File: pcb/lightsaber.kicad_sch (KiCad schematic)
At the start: 66 parts, among them IC1 BMI055, J1 2012670005, J2 Screw_Terminal_01x05, J3 ESP32 Prog, J4 ESP32 JTAG, J5 Conn_01x02, J6 Conn_01x06, Q1 PMOS, Q2 NPN, SW1 SW_Push, SW2 SW_Push, U1 ME6211A33PG-N, U2 ESP32-S3-WROOM-1, U3 ACS725xLCTR-10AU, U4 BQ21040DBVR, U5 5994, U6 MAX17048G+T10, U7 AHT20

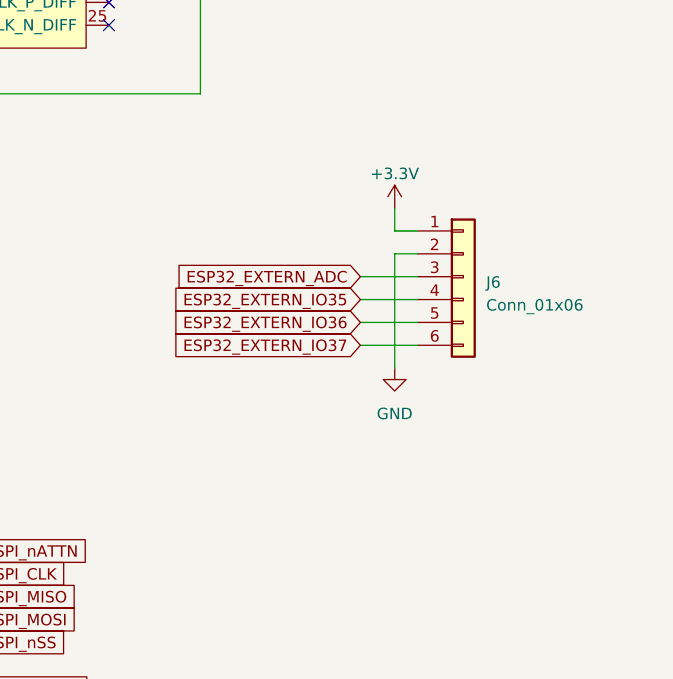
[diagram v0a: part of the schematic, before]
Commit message: Tidying up traces
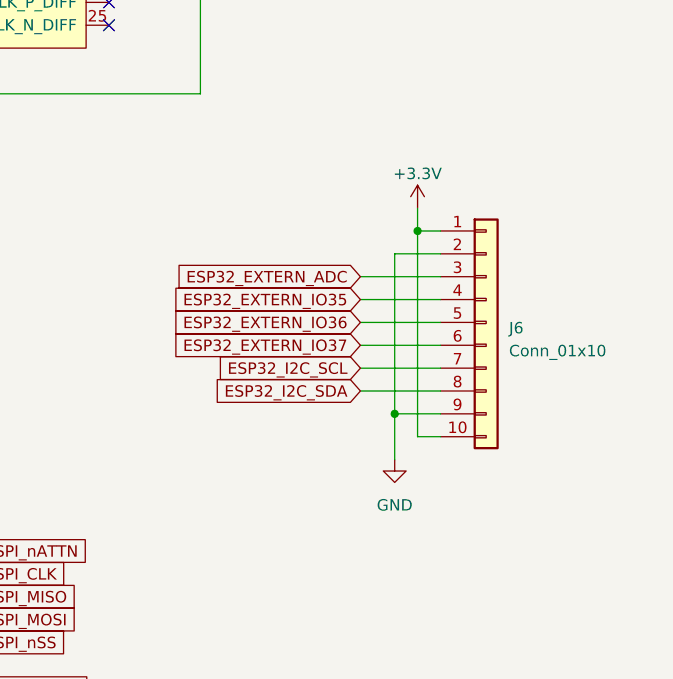
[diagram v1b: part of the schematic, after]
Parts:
- removed J6: Conn_01x06, Connector_PinHeader_2.54mm:PinHeader_1x06_P2.54mm_Vertical, symbol Connector_Generic:Conn_01x06
- added J6: Conn_01x10, Connector_PinHeader_2.54mm:PinHeader_1x10_P2.54mm_Vertical, symbol Connector_Generic:Conn_01x10
- SW1, SW2: LCSC C318884 -> C492878
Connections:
- net +3.3V: now also J6.1 (Pin_1), J6.10 (Pin_10)
- net ESP32_EXTERN_ADC: now also J6.3 (Pin_3)
- net ESP32_EXTERN_IO35: now also J6.4 (Pin_4)
- net ESP32_EXTERN_IO36: now also J6.5 (Pin_5)
- net ESP32_EXTERN_IO37: now also J6.6 (Pin_6)
- net ESP32_I2C_SCL: now also J6.7 (Pin_7)
- net ESP32_I2C_SDA: now also J6.8 (Pin_8)
- net GND: now also J6.2 (Pin_2), J6.9 (Pin_9)
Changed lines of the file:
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@@
   (junction (at 118.11 201.93) (diameter 0) (color 0 0 0 0)
   )
+  (junction (at 544.83 158.75) (diameter 0) (color 0 0 0 0)
+  )
   (junction (at 21.59 44.45) (diameter 0) (color 0 0 0 0)
   )
@@
   (junction (at 387.35 44.45) (diameter 0) (color 0 0 0 0)
   )
+  (junction (at 547.37 138.43) (diameter 0) (color 0 0 0 0)
+  )
   (junction (at 466.09 212.09) (diameter 0) (color 0 0 0 0)
   )
@@
     (stroke (width 0) (type default))
   )
-  (wire (pts (xy 544.83 138.43) (xy 547.37 138.43))
+  (wire (pts (xy 547.37 138.43) (xy 549.91 138.43))
     (stroke (width 0) (type default))
   )
@@
     (stroke (width 0) (type default))
   )
-  (wire (pts (xy 544.83 140.97) (xy 544.83 153.67))
+  (wire (pts (xy 544.83 140.97) (xy 544.83 158.75))
     (stroke (width 0) (type default))
   )
@@
     (stroke (width 0) (type default))
   )
-  (wire (pts (xy 544.83 140.97) (xy 547.37 140.97))
+  (wire (pts (xy 544.83 140.97) (xy 549.91 140.97))
     (stroke (width 0) (type default))
   )
@@
     (stroke (width 0) (type default))
   )
+  (wire (pts (xy 541.02 153.67) (xy 549.91 153.67))
+    (stroke (width 0) (type default))
+  )
   (wire (pts (xy 476.25 209.55) (xy 476.25 212.09))
     (stroke (width 0) (type default))
@@
     (stroke (width 0) (type default))
   )
+  (wire (pts (xy 549.91 161.29) (xy 547.37 161.29))
+    (stroke (width 0) (type default))
+  )
   (wire (pts (xy 114.3 261.62) (xy 111.76 261.62))
     (stroke (width 0) (type default))
@@
     (stroke (width 0) (type default))
   )
+  (wire (pts (xy 544.83 158.75) (xy 544.83 163.83))
+    (stroke (width 0) (type default))
+  )
   (wire (pts (xy 104.14 130.81) (xy 107.95 130.81))
     (stroke (width 0) (type default))
@@
     (stroke (width 0) (type default))
   )
-  (wire (pts (xy 541.02 146.05) (xy 547.37 146.05))
+  (wire (pts (xy 541.02 146.05) (xy 549.91 146.05))
     (stroke (width 0) (type default))
   )
@@
     (stroke (width 0) (type default))
   )
-  (wire (pts (xy 541.02 143.51) (xy 547.37 143.51))
+  (wire (pts (xy 541.02 143.51) (xy 549.91 143.51))
     (stroke (width 0) (type default))
   )
@@
     (stroke (width 0) (type default))
   )
+  (wire (pts (xy 547.37 161.29) (xy 547.37 138.43))
+    (stroke (width 0) (type default))
+  )
   (wire (pts (xy 140.97 125.73) (xy 140.97 115.57))
     (stroke (width 0) (type default))
@@
     (stroke (width 0) (type default))
   )
+  (wire (pts (xy 541.02 156.21) (xy 549.91 156.21))
+    (stroke (width 0) (type default))
+  )
   (wire (pts (xy 58.42 123.19) (xy 60.96 123.19))
     (stroke (width 0) (type default))
@@
     (stroke (width 0) (type default))
   )
+  (wire (pts (xy 544.83 158.75) (xy 549.91 158.75))
+    (stroke (width 0) (type default))
+  )
   (wire (pts (xy 513.08 90.17) (xy 528.32 90.17))
     (stroke (width 0) (type default))
@@
     (stroke (width 0) (type default))
   )
-  (wire (pts (xy 541.02 151.13) (xy 547.37 151.13))
+  (wire (pts (xy 541.02 151.13) (xy 549.91 151.13))
     (stroke (width 0) (type default))
   )
@@
     (stroke (width 0) (type default))
   )
-  (wire (pts (xy 541.02 148.59) (xy 547.37 148.59))
+  (wire (pts (xy 541.02 148.59) (xy 549.91 148.59))
     (stroke (width 0) (type default))
   )
@@
     (stroke (width 0) (type default))
   )
-  (wire (pts (xy 544.83 135.89) (xy 544.83 138.43))
+  (wire (pts (xy 547.37 135.89) (xy 547.37 138.43))
     (stroke (width 0) (type default))
   )
@@
     )
   )
+  (global_label "ESP32_I2C_SDA" (shape input) (at 541.02 156.21 180) (fields_autoplaced)
+    (effects (font (size 1.27 1.27)) (justify right))
+    (property "Intersheetrefs" "${INTERSHEET_REFS}" (at 523.4791 156.21 0)
+      (effects (font (size 1.27 1.27)) (justify right) hide)
+    )
+  )
   (global_label "ESP32_BMI_GYRO_2" (shape input) (at 528.32 77.47 0) (fields_autoplaced)
     (effects (font (size 1.27 1.27)) (justify left))
@@
     )
   )
+  (global_label "ESP32_I2C_SCL" (shape input) (at 541.02 153.67 180) (fields_autoplaced)
+    (effects (font (size 1.27 1.27)) (justify right))
+    (property "Intersheetrefs" "${INTERSHEET_REFS}" (at 523.5396 153.67 0)
+      (effects (font (size 1.27 1.27)) (justify right) hide)
+    )
+  )
   (global_label "ESP32_EXTERN_IO37" (shape input) (at 416.56 115.57 180) (fields_autoplaced)
     (effects (font (size 1.27 1.27)) (justify right))
@@
     )
   )
-  (symbol (lib_id "power:+3.3V") (at 544.83 135.89 0) (unit 1)
+  (symbol (lib_id "power:+3.3V") (at 547.37 135.89 0) (unit 1)
     (in_bom yes) (on_board yes) (dnp no) (fields_autoplaced)
-    (property "Reference" "#PWR039" (at 544.83 139.7 0)
+    (property "Reference" "#PWR039" (at 547.37 139.7 0)
       (effects (font (size 1.27 1.27)) hide)
     )
-    (property "Value" "+3.3V" (at 544.83 132.08 0)
+    (property "Value" "+3.3V" (at 547.37 132.08 0)
       (effects (font (size 1.27 1.27)))
     )
-    (property "Footprint" "" (at 544.83 135.89 0)
+    (property "Footprint" "" (at 547.37 135.89 0)
       (effects (font (size 1.27 1.27)) hide)
     )
-    (property "Datasheet" "" (at 544.83 135.89 0)
+    (property "Datasheet" "" (at 547.37 135.89 0)
       (effects (font (size 1.27 1.27)) hide)
     )
@@
     )
   )
-  (symbol (lib_id "power:GND") (at 544.83 153.67 0) (unit 1)
+  (symbol (lib_id "power:GND") (at 544.83 163.83 0) (unit 1)
     (in_bom yes) (on_board yes) (dnp no) (fields_autoplaced)
-    (property "Reference" "#PWR050" (at 544.83 160.02 0)
+    (property "Reference" "#PWR050" (at 544.83 170.18 0)
       (effects (font (size 1.27 1.27)) hide)
     )
-    (property "Value" "GND" (at 544.83 158.75 0)
+    (property "Value" "GND" (at 544.83 168.91 0)
       (effects (font (size 1.27 1.27)))
     )
-    (property "Footprint" "" (at 544.83 153.67 0)
+    (property "Footprint" "" (at 544.83 163.83 0)
       (effects (font (size 1.27 1.27)) hide)
     )
-    (property "Datasheet" "" (at 544.83 153.67 0)
+    (property "Datasheet" "" (at 544.83 163.83 0)
       (effects (font (size 1.27 1.27)) hide)
     )
@@
       (effects (font (size 1.27 1.27)) hide)
     )
-    (property "LCSC" "C318884" (at 189.23 280.67 0)
+    (property "LCSC" "C492878" (at 189.23 280.67 0)
+      (effects (font (size 1.27 1.27)) hide)
+    )
+    (property "Field" "" (at 189.23 280.67 90)
       (effects (font (size 1.27 1.27)) hide)
     )
@@
     )
   )
+  (symbol (lib_id "Connector_Generic:Conn_01x10") (at 554.99 148.59 0) (unit 1)
+    (in_bom yes) (on_board yes) (dnp no) (fields_autoplaced)
+    (property "Reference" "J6" (at 557.53 149.225 0)
+      (effects (font (size 1.27 1.27)) (justify left))
+    )
+    (property "Value" "Conn_01x10" (at 557.53 151.765 0)
+      (effects (font (size 1.27 1.27)) (justify left))
+    )
+    (property "Footprint" "Connector_PinHeader_2.54mm:PinHeader_1x10_P2.54mm_Vertical" (at 554.99 148.59 0)
+      (effects (font (size 1.27 1.27)) hide)
+    )
+    (property "Datasheet" "~" (at 554.99 148.59 0)
+      (effects (font (size 1.27 1.27)) hide)
+    )
+    (pin "1")
+    (pin "10")
+    (pin "2")
+    (pin "3")
+    (pin "4")
+    (pin "5")
+    (pin "6")
+    (pin "7")
+    (pin "8")
+    (pin "9")
+    (instances
+      (project "lightsaber"
+        (path "/480b6f8b-587f-4642-8a87-aec0c171ba44"
+          (reference "J6") (unit 1)
+        )
+      )
+    )
+  )
   (symbol (lib_id "power:+3.3V") (at 316.23 252.73 0) (unit 1)
     (in_bom yes) (on_board yes) (dnp no) (fields_autoplaced)
@@
     )
   )
-  (symbol (lib_id "Connector_Generic:Conn_01x06") (at 552.45 143.51 0) (unit 1)
-    (in_bom yes) (on_board yes) (dnp no) (fields_autoplaced)
-    (property "Reference" "J6" (at 554.99 144.145 0)
-      (effects (font (size 1.27 1.27)) (justify left))
-    )
-    (property "Value" "Conn_01x06" (at 554.99 146.685 0)
-      (effects (font (size 1.27 1.27)) (justify left))
-    )
-    (property "Footprint" "Connector_PinHeader_2.54mm:PinHeader_1x06_P2.54mm_Vertical" (at 552.45 143.51 0)
-      (effects (font (size 1.27 1.27)) hide)
-    )
-    (property "Datasheet" "~" (at 552.45 143.51 0)
-      (effects (font (size 1.27 1.27)) hide)
-    )
-    (pin "1")
-    (pin "2")
-    (pin "3")
-    (pin "4")
-    (pin "5")
-    (pin "6")
-    (instances
-      (project "lightsaber"
-        (path "/480b6f8b-587f-4642-8a87-aec0c171ba44"
-          (reference "J6") (unit 1)
-        )
-      )
-    )
-  )
   (symbol (lib_id "Device:C_Small") (at 140.97 128.27 0) (unit 1)
     (in_bom yes) (on_board yes) (dnp no) (fields_autoplaced)
@@
       (effects (font (size 1.27 1.27)) hide)
     )
-    (property "LCSC" "C318884" (at 179.07 280.67 0)
+    (property "LCSC" "C492878" (at 179.07 280.67 0)
       (effects (font (size 1.27 1.27)) hide)
     )
